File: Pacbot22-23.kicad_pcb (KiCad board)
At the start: 2 copper layers, 76.2 x 76.2 mm, 0 parts

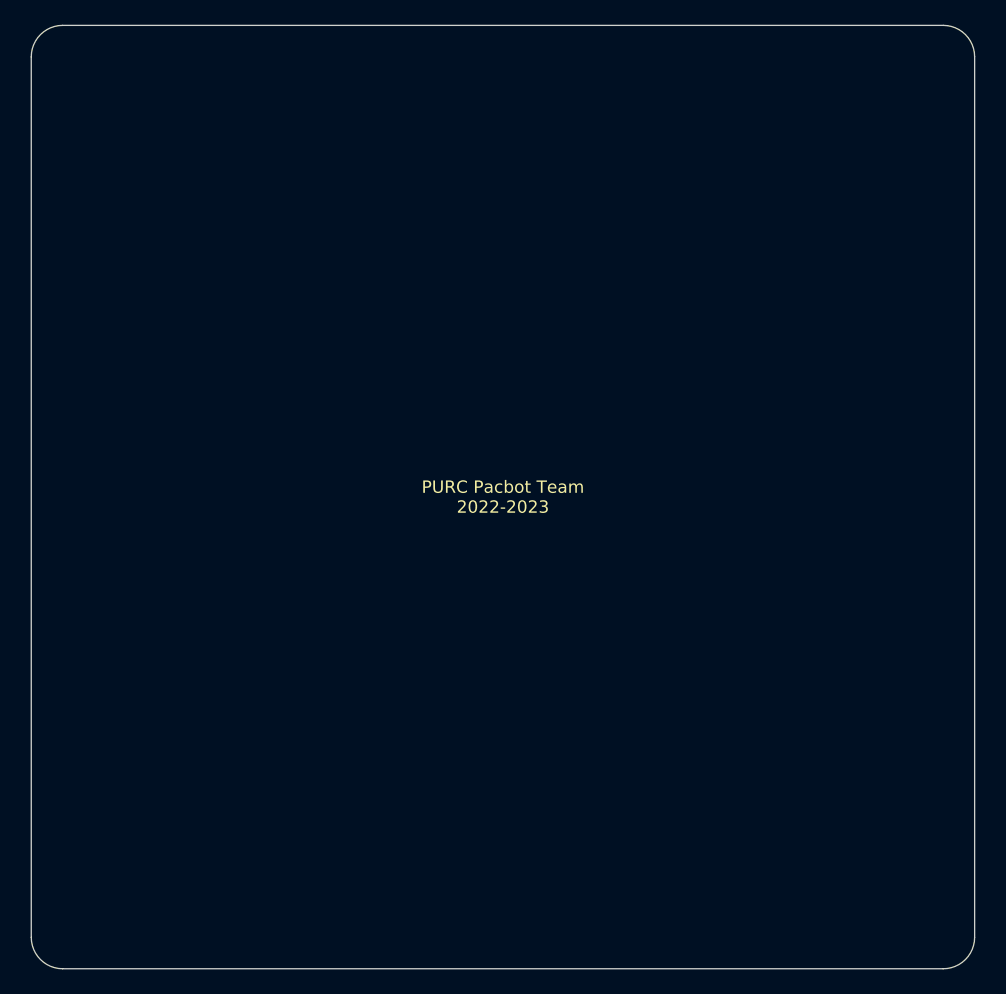
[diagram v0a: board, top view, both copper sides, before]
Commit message: Pushing PCB
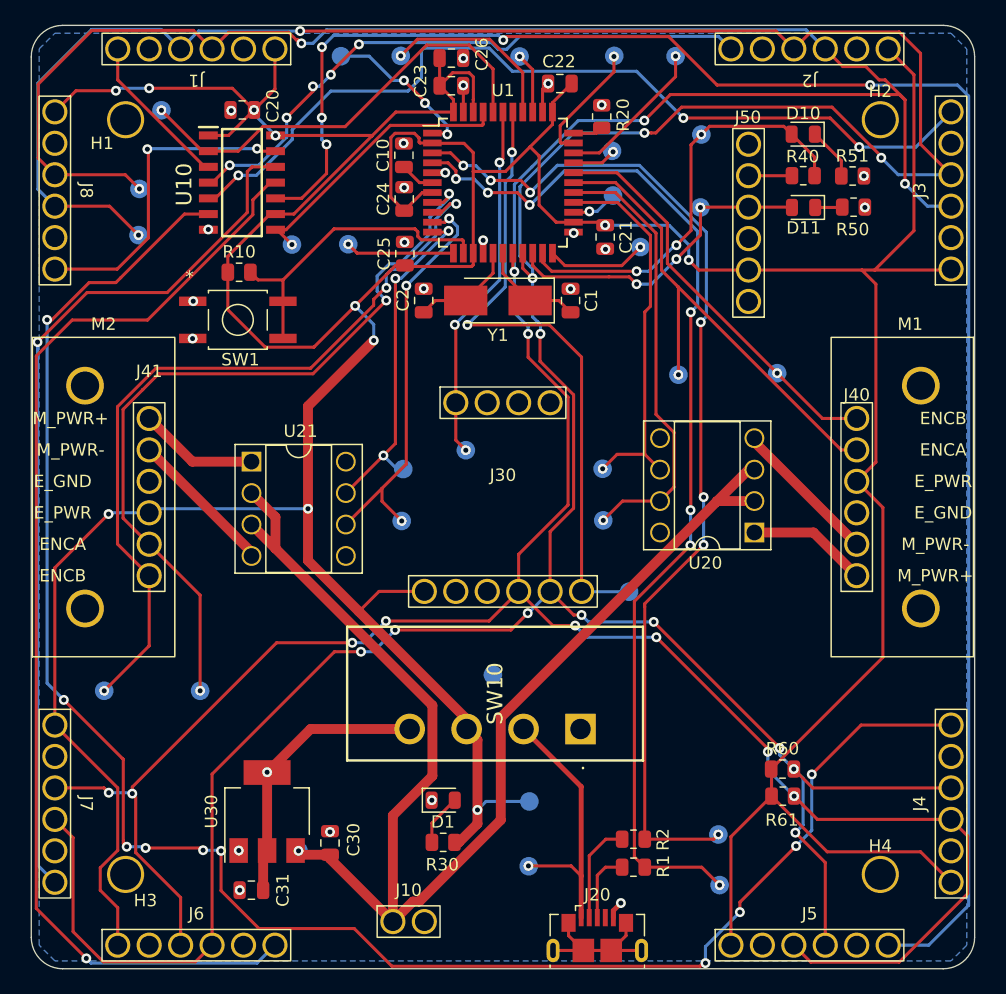
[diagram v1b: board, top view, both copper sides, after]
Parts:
- added C1: 15pF, Capacitor_SMD:C_0805_2012Metric, F.Cu at (119.8, 73.0)
- added C10: 1uF, Capacitor_SMD:C_0805_2012Metric, F.Cu at (106.3, 61.3)
- added C2: 15pF, Capacitor_SMD:C_0805_2012Metric, F.Cu at (107.9, 73.0)
- added C20: 0.1uF, Capacitor_SMD:C_0805_2012Metric, F.Cu at (93.2, 57.6)
- added C21: 0.1uF, Capacitor_SMD:C_0805_2012Metric, F.Cu at (122.6, 67.9)
- added C22: 0.1uF, Capacitor_SMD:C_0805_2012Metric, F.Cu at (118.9, 55.5)
- added C23: 0.1uF, Capacitor_SMD:C_0805_2012Metric, F.Cu at (110.1, 55.7)
- added C24: 0.1uF, Capacitor_SMD:C_0805_2012Metric, F.Cu at (106.3, 64.8)
- added C25: 0.1uF, Capacitor_SMD:C_0805_2012Metric, F.Cu at (106.4, 69.2)
- added C26: 10uF, Capacitor_SMD:C_0805_2012Metric, F.Cu at (110.1, 53.4)
- added C30: 10uF, Capacitor_SMD:C_0805_2012Metric, F.Cu at (100.3, 116.8)
- added C31: 22uF, Capacitor_SMD:C_0805_2012Metric, F.Cu at (94.0, 120.7)
- added D1: LED_Small, Diode_SMD:D_0805_2012Metric, F.Cu at (109.5, 113.4)
- added D10: LED_Small, Diode_SMD:D_0805_2012Metric, F.Cu at (138.6, 59.6)
- added D11: LED_Small, Diode_SMD:D_0805_2012Metric, F.Cu at (138.6, 65.5)
- added H1: MountingHole, MountingHole:MountingHole_2.5mm_Pad, F.Cu at (83.8, 58.4)
- added H2: MountingHole, MountingHole:MountingHole_2.5mm_Pad, F.Cu at (144.8, 58.4)
- added H3: MountingHole, MountingHole:MountingHole_2.5mm_Pad, F.Cu at (83.8, 119.4)
- added H4: MountingHole, MountingHole:MountingHole_2.5mm_Pad, F.Cu at (144.8, 119.4)
- added J1: VL6180X, CustomFootprints:VL6180X, F.Cu at (89.5, 52.7)
- added J10: Screw_Terminal_01x02, CustomFootprints:POWER_TERM, F.Cu at (106.7, 123.2)
- added J2: VL6180X, CustomFootprints:VL6180X, F.Cu at (139.1, 52.7)
- added J20: USB_B_Micro, Connector_USB:USB_Micro-B_GCT_USB3076-30-A, F.Cu at (121.9, 124.3)
- added J3: VL6180X, CustomFootprints:VL6180X, F.Cu at (150.5, 64.1)
- added J30: BNO-055, CustomFootprints:BNO055, F.Cu at (114.3, 87.6)
- added J4: VL6180X, CustomFootprints:VL6180X, F.Cu at (150.5, 113.7)
- added J40: 6V_DC_Motor, CustomFootprints:6V_DC_Motor, F.Cu at (142.9, 86.4)
- added J41: 6V_DC_Motor, CustomFootprints:6V_DC_Motor, F.Cu at (85.7, 91.4)
- added J5: VL6180X, CustomFootprints:VL6180X, F.Cu at (139.1, 125.1)
- added J50: HC-05, CustomFootprints:HC-05, F.Cu at (134.1, 76.9)
- added J6: VL6180X, CustomFootprints:VL6180X, F.Cu at (89.5, 125.1)
- added J7: VL6180X, CustomFootprints:VL6180X, F.Cu at (78.1, 113.7)
- added J8: VL6180X, CustomFootprints:VL6180X, F.Cu at (78.1, 64.1)
- added M1: M1_Mount, CustomFootprints:Motor_Mount, F.Cu at (148.1, 88.9)
- added M2: M2_Mount, CustomFootprints:Motor_Mount, F.Cu at (80.5, 88.9)
- added R1: 22r, Resistor_SMD:R_0805_2012Metric, F.Cu at (124.8, 118.8)
- added R10: 10k, Resistor_SMD:R_0805_2012Metric, F.Cu at (93.0, 70.7)
- added R2: 22r, Resistor_SMD:R_0805_2012Metric, F.Cu at (124.8, 116.5)
- added R20: 10k, Resistor_SMD:R_0805_2012Metric, F.Cu at (122.3, 58.2)
- added R30: 1k, Resistor_SMD:R_0805_2012Metric, F.Cu at (109.5, 116.8)
- added R40: 100r, Resistor_SMD:R_0805_2012Metric, F.Cu at (138.6, 62.9)
- added R50: 1k, Resistor_SMD:R_0805_2012Metric, F.Cu at (142.6, 65.5)
- added R51: 1k, Resistor_SMD:R_0805_2012Metric, F.Cu at (142.5, 63.0)
- added R60: 2k2, Resistor_SMD:R_0805_2012Metric, F.Cu at (136.9, 110.9)
- added R61: 2k2, Resistor_SMD:R_0805_2012Metric, F.Cu at (136.9, 113.1)
- added SW1: SW_Push_Dual, CustomFootprints:TL3305AF260QG, F.Cu at (92.9, 74.6)
- added SW10: L103011MS02Q, CustomFootprints:L103011MS02Q, F.Cu at (120.6, 107.6)
- added TP_5V_1: TestPoint, TestPoint:TestPoint_Pad_D1.5mm, B.Cu at (116.4, 113.5)
- added TP_B6: TestPoint, TestPoint:TestPoint_Pad_D1.5mm, B.Cu at (123.1, 60.9)
- added TP_B7: TestPoint, TestPoint:TestPoint_Pad_D1.5mm, B.Cu at (101.8, 68.5)
- added TP_C6: TestPoint, TestPoint:TestPoint_Pad_D1.5mm, B.Cu at (128.2, 53.3)
- added TP_C7: TestPoint, TestPoint:TestPoint_Pad_D1.5mm, B.Cu at (123.3, 53.3)
- added TP_D+_1: TestPoint, TestPoint:TestPoint_Pad_D1.5mm, B.Cu at (131.8, 120.2)
- added TP_D-_1: TestPoint, TestPoint:TestPoint_Pad_D1.5mm, B.Cu at (131.7, 116.2)
- added TP_D4: TestPoint, TestPoint:TestPoint_Pad_D1.5mm, B.Cu at (123.2, 64.5)
- added TP_D5: TestPoint, TestPoint:TestPoint_Pad_D1.5mm, B.Cu at (125.4, 68.7)
- added TP_E6: TestPoint, TestPoint:TestPoint_Pad_D1.5mm, B.Cu at (101.2, 53.3)
- added TP_ENC11: TestPoint, TestPoint:TestPoint_Pad_D1.5mm, B.Cu at (128.5, 79.0)
- added TP_ENC12: TestPoint, TestPoint:TestPoint_Pad_D1.5mm, B.Cu at (136.4, 78.9)
- added TP_ENC21: TestPoint, TestPoint:TestPoint_Pad_D1.5mm, B.Cu at (89.8, 104.5)
- added TP_ENC22: TestPoint, TestPoint:TestPoint_Pad_D1.5mm, B.Cu at (82.1, 104.5)
- added TP_F0: TestPoint, TestPoint:TestPoint_Pad_D1.5mm, B.Cu at (97.3, 68.5)
- added TP_F1: TestPoint, TestPoint:TestPoint_Pad_D1.5mm, B.Cu at (86.7, 57.7)
- added TP_F4: TestPoint, TestPoint:TestPoint_Pad_D1.5mm, B.Cu at (111.3, 85.1)
- added TP_F5: TestPoint, TestPoint:TestPoint_Pad_D1.5mm, B.Cu at (124.5, 96.5)
- added TP_F6: TestPoint, TestPoint:TestPoint_Pad_D1.5mm, B.Cu at (106.0, 53.3)
- added TP_F7: TestPoint, TestPoint:TestPoint_Pad_D1.5mm, B.Cu at (115.6, 53.3)
- added TP_GND_1: TestPoint, TestPoint:TestPoint_Pad_D1.5mm, B.Cu at (113.5, 103.3)
- added TP_M11: TestPoint, TestPoint:TestPoint_Pad_D1.5mm, B.Cu at (122.4, 86.6)
- added TP_M12: TestPoint, TestPoint:TestPoint_Pad_D1.5mm, B.Cu at (122.4, 90.8)
- added TP_M21: TestPoint, TestPoint:TestPoint_Pad_D1.5mm, B.Cu at (106.1, 90.8)
- added TP_M22: TestPoint, TestPoint:TestPoint_Pad_D1.5mm, B.Cu at (106.2, 86.6)
- added TP_RX_1: TestPoint, TestPoint:TestPoint_Pad_D1.5mm, B.Cu at (130.3, 65.5)
- added TP_SCL_1: TestPoint, TestPoint:TestPoint_Pad_D1.5mm, B.Cu at (84.9, 64.0)
- added TP_SDA_1: TestPoint, TestPoint:TestPoint_Pad_D1.5mm, B.Cu at (84.9, 67.7)
- added TP_TX_1: TestPoint, TestPoint:TestPoint_Pad_D1.5mm, B.Cu at (130.3, 59.6)
- added TP_VBAT_1: TestPoint, TestPoint:TestPoint_Pad_D1.5mm, B.Cu at (97.8, 117.5)
- added TP_VREG_1: TestPoint, TestPoint:TestPoint_Pad_D1.5mm, B.Cu at (95.2, 111.1)
- added TP_VUSB_1: TestPoint, TestPoint:TestPoint_Pad_D1.5mm, B.Cu at (116.4, 118.7)
- added U1: ATmega32U4-A, Package_QFP:TQFP-44_10x10mm_P0.8mm, F.Cu at (114.3, 63.5)
- added U10: SN74HCS264DR, CustomFootprints:SOIC127P600X175-14N, F.Cu at (93.2, 63.5)
- added U20: L9110_HBridge, CustomFootprints:Adafruit_L9110_HBridge, F.Cu at (130.8, 95.0)
- added U21: L9110_HBridge, CustomFootprints:Adafruit_L9110_HBridge, F.Cu at (97.8, 82.8)
- added U30: AZ1117I-5.0, Package_TO_SOT_SMD:SOT-223-3_TabPin2, F.Cu at (95.2, 114.3)
- added Y1: 16Mhz, Crystal:Crystal_SMD_5032-2Pin_5.0x3.2mm_HandSoldering, F.Cu at (113.9, 73.0)
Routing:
- net +5V: track 0.00 -> 398.1 mm, vias 0 -> 11
- net SDA: track 0.00 -> 307.7 mm, vias 0 -> 14
- net SCL: track 0.00 -> 301.1 mm, vias 0 -> 14
- net XS4: track 0.00 -> 146.2 mm, vias 0 -> 10
- net XS5: track 0.00 -> 143.4 mm, vias 0 -> 5
- net +8V: track 0.00 -> 107.4 mm, vias 0 -> 1
- net XS6: track 0.00 -> 92.2 mm, vias 0 -> 1
- net D+: track 0.00 -> 86.9 mm, vias 0 -> 7
- net D-: track 0.00 -> 84.1 mm, vias 0 -> 7
- net XS3: track 0.00 -> 71.2 mm, vias 0 -> 3
- net XS7: track 0.00 -> 71.2 mm, vias 0 -> 1
- net ENC21: track 0.00 -> 63.8 mm, vias 0 -> 3
- net ENC22: track 0.00 -> 63.6 mm, vias 0 -> 3
- net BNO_RST: track 0.00 -> 51.8 mm, vias 0 -> 2
- net XS2: track 0.00 -> 49.2 mm, vias 0 -> 5
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- added copper zone on B.Cu, net GND
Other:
- board text removed: "PURC Pacbot Team 2022-2023"
